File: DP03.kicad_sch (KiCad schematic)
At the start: 21 parts

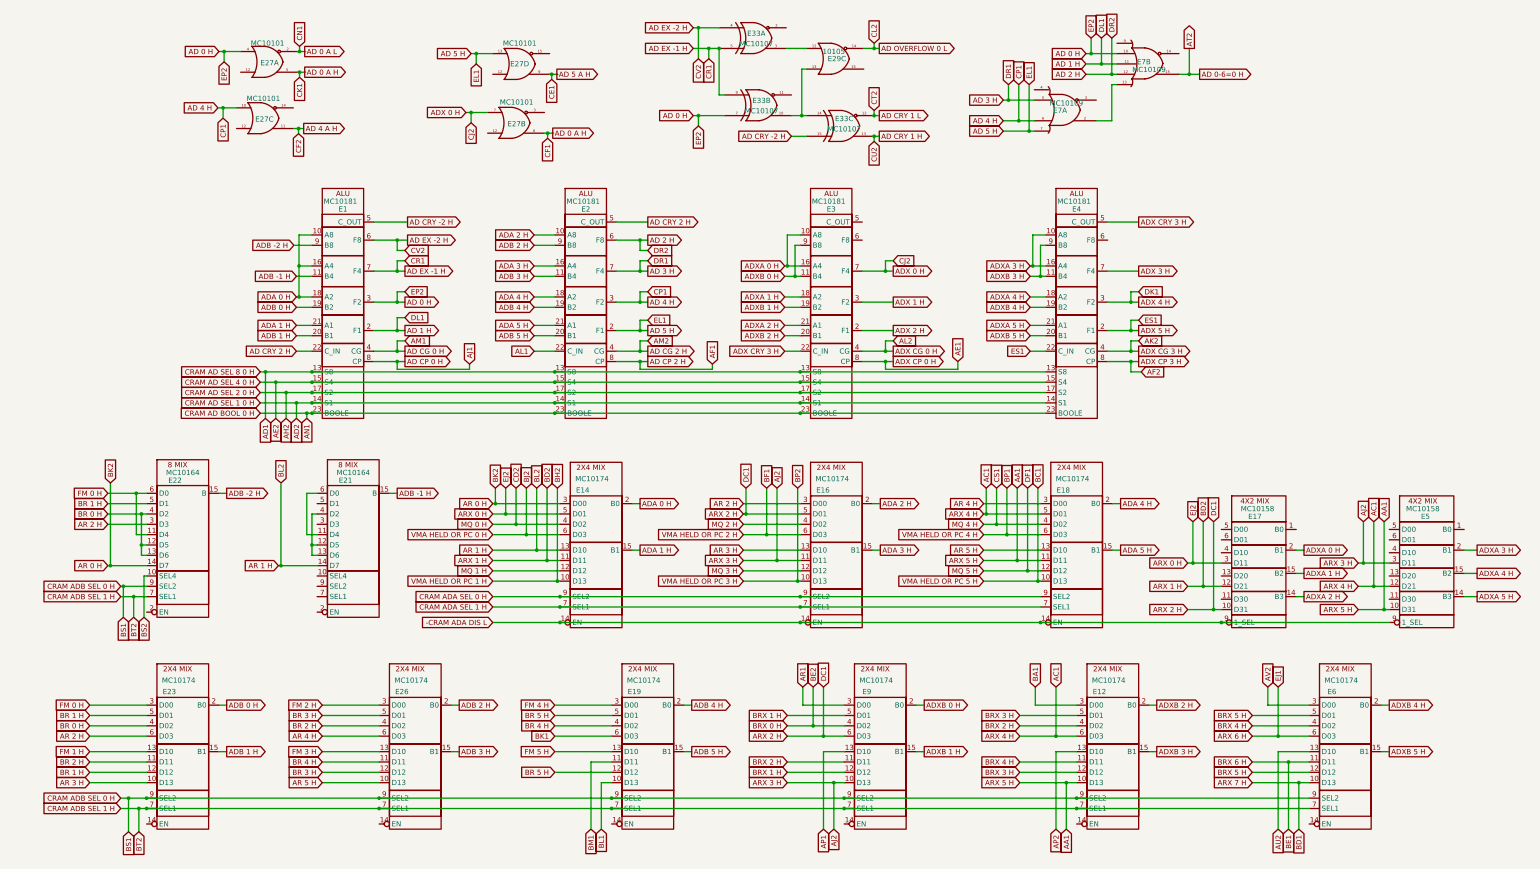
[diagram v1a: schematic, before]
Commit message: checkpoint
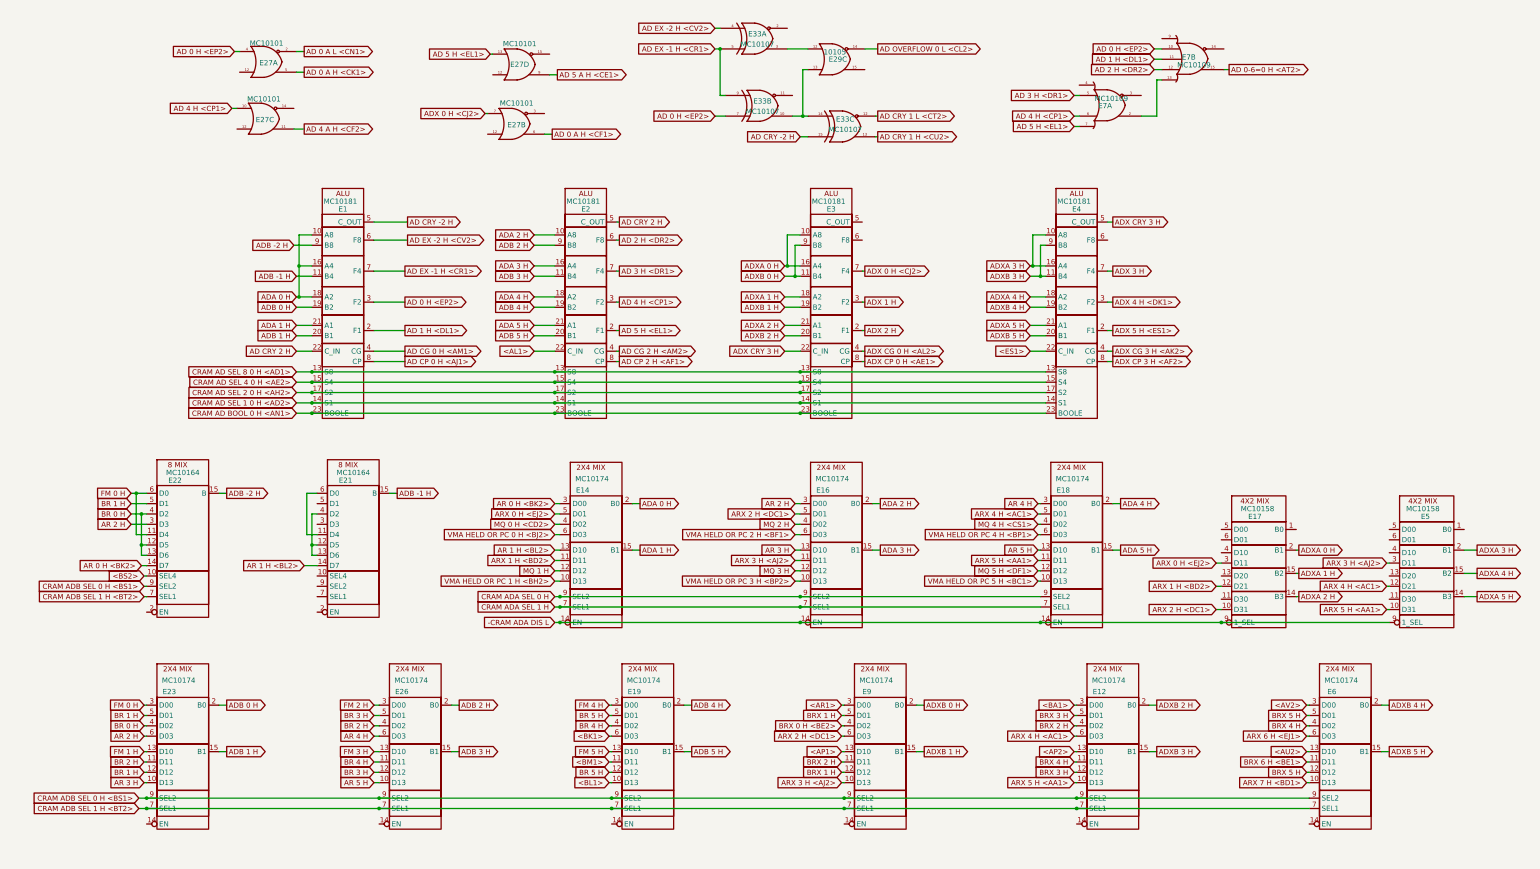
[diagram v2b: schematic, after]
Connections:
- net AA1 renamed ARX 5 H <AA1>
- net AC1 renamed ARX 4 H <AC1>
- net AD 0 A H renamed AD 0 A H <CF1>
- net AD 0 A H <CF1>: no longer E27.5 (Aout)
- net AD 0 A L renamed AD 0 A L <CN1>
- net AD 0 H renamed AD 0 H <EP2>
- net AD 0-6=0 H renamed AD 0-6=0 H <AT2>
- net AD 1 H renamed AD 1 H <DL1>
- net AD 2 H renamed AD 2 H <DR2>
- net AD 3 H renamed AD 3 H <DR1>
- net AD 4 A H renamed AD 4 A H <CF2>
- net AD 4 H renamed AD 4 H <CP1>
- net AD 5 A H renamed AD 5 A H <CE1>
- net AD 5 H renamed AD 5 H <EL1>
- net AD CG 0 H renamed AD CG 0 H <AM1>
- net AD CG 2 H renamed AD CG 2 H <AM2>
- net AD CP 0 H renamed AD CP 0 H <AJ1>
- net AD CP 2 H renamed AD CP 2 H <AF1>
- net AD CRY 1 H renamed AD CRY 1 H <CU2>
- net AD CRY 1 L renamed AD CRY 1 L <CT2>
- net AD EX -1 H renamed AD EX -1 H <CR1>
- net AD EX -2 H renamed AD EX -2 H <CV2>
- net AD OVERFLOW 0 L renamed AD OVERFLOW 0 L <CL2>
- net AD1 renamed CRAM AD SEL 8 0 H <AD1>
- net AD2 renamed CRAM AD SEL 1 0 H <AD2>
- net ADX 0 H renamed ADX 0 H <CJ2>
- net ADX 4 H renamed ADX 4 H <DK1>
- net ADX 5 H renamed <ES1>
- net <ES1>: no longer E4.2 (F1)
- net ADX CG 0 H renamed ADX CG 0 H <AL2>
- net ADX CG 3 H renamed ADX CG 3 H <AK2>
- net ADX CP 0 H renamed ADX CP 0 H <AE1>
- net ADX CP 3 H renamed ADX CP 3 H <AF2>
- net AE2 renamed CRAM AD SEL 4 0 H <AE2>
- net AH2 renamed CRAM AD SEL 2 0 H <AH2>
- net AJ2 renamed ARX 3 H <AJ2>
- net AL1 renamed <AL1>
- net AN1 renamed CRAM AD BOOL 0 H <AN1>
- net AP1 renamed <AP1>
- net AP2 renamed <AP2>
- net AR 0 H renamed AR 0 H <BK2>
- net AR 1 H renamed AR 1 H <BL2>
- net AR1 renamed <AR1>
- net ARX 0 H renamed ARX 0 H <EJ2>
- net ARX 1 H renamed ARX 1 H <BD2>
- net ARX 2 H renamed ARX 2 H <DC1>
- net ARX 6 H renamed ARX 6 H <EJ1>
- net ARX 7 H renamed ARX 7 H <BD1>
- net AU2 renamed <AU2>
- net AV2 renamed <AV2>
- net BA1 renamed <BA1>
- net BC1 renamed VMA HELD OR PC 5 H <BC1>
- net BE1 renamed BRX 6 H <BE1>
- net BE2 renamed BRX 0 H <BE2>
- net BF1 renamed VMA HELD OR PC 2 H <BF1>
- net BH2 renamed VMA HELD OR PC 1 H <BH2>
- net BJ2 renamed VMA HELD OR PC 0 H <BJ2>
- net BK1 renamed <BK1>
- net BL1 renamed <BL1>
- net BM1 renamed <BM1>
- net BP1 renamed VMA HELD OR PC 4 H <BP1>
- net BP2 renamed VMA HELD OR PC 3 H <BP2>
- net BS1 renamed CRAM ADB SEL 0 H <BS1>
- net BS2 renamed <BS2>
- net BT2 renamed CRAM ADB SEL 1 H <BT2>
- net CD2 renamed MQ 0 H <CD2>
- net CS1 renamed MQ 4 H <CS1>
- net DF1 renamed MQ 5 H <DF1>
- new net AD 0 A H <CK1>: E27.5 (Aout)
- new net ADX 5 H <ES1>: E4.2 (F1)
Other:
- moved on the sheet: E7A, E7B
